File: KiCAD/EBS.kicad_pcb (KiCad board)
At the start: 2 copper layers, 44.4 x 27.4 mm, 21 parts, among them Q1 BC547, Q2 BC557

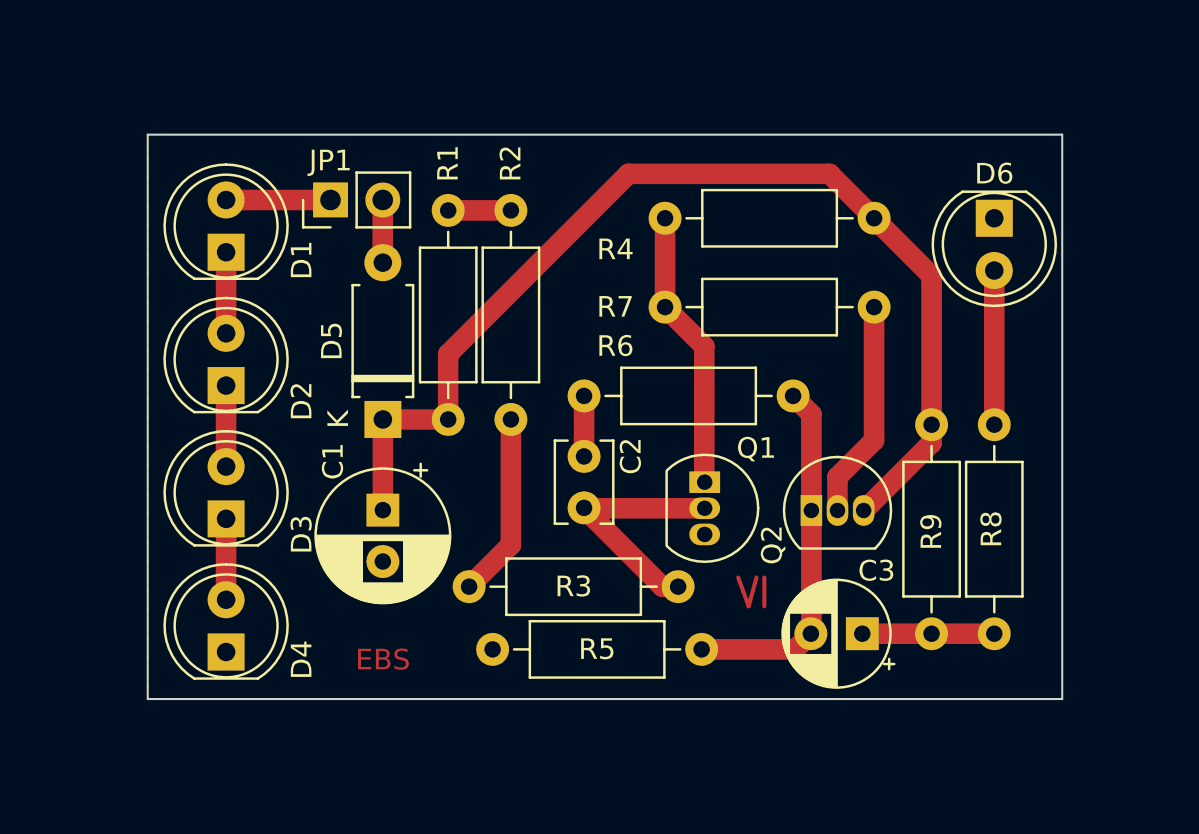
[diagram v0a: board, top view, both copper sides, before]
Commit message: Update
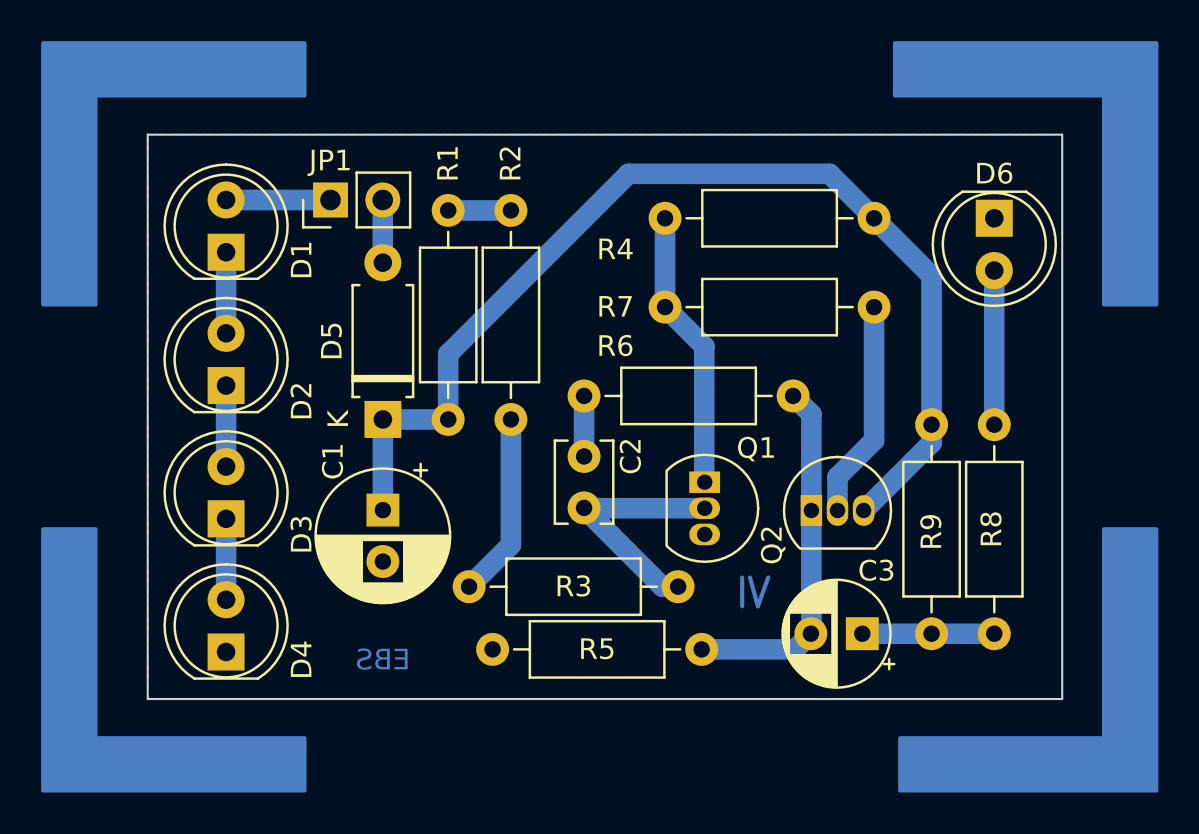
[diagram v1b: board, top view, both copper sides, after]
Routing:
- added copper zone on B.Cu, net GND
- removed copper zone on F.Cu, net GND
